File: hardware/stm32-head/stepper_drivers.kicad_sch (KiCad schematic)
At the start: 74 parts, among them J10 STEPPER4, J17 STEPPER6, J18 STEPPER5, J7 STEPPER1, J8 STEPPER2, J9 STEPPER3, U10 STSPIN220, U11 STSPIN220, U12 STSPIN220, U9 STSPIN220

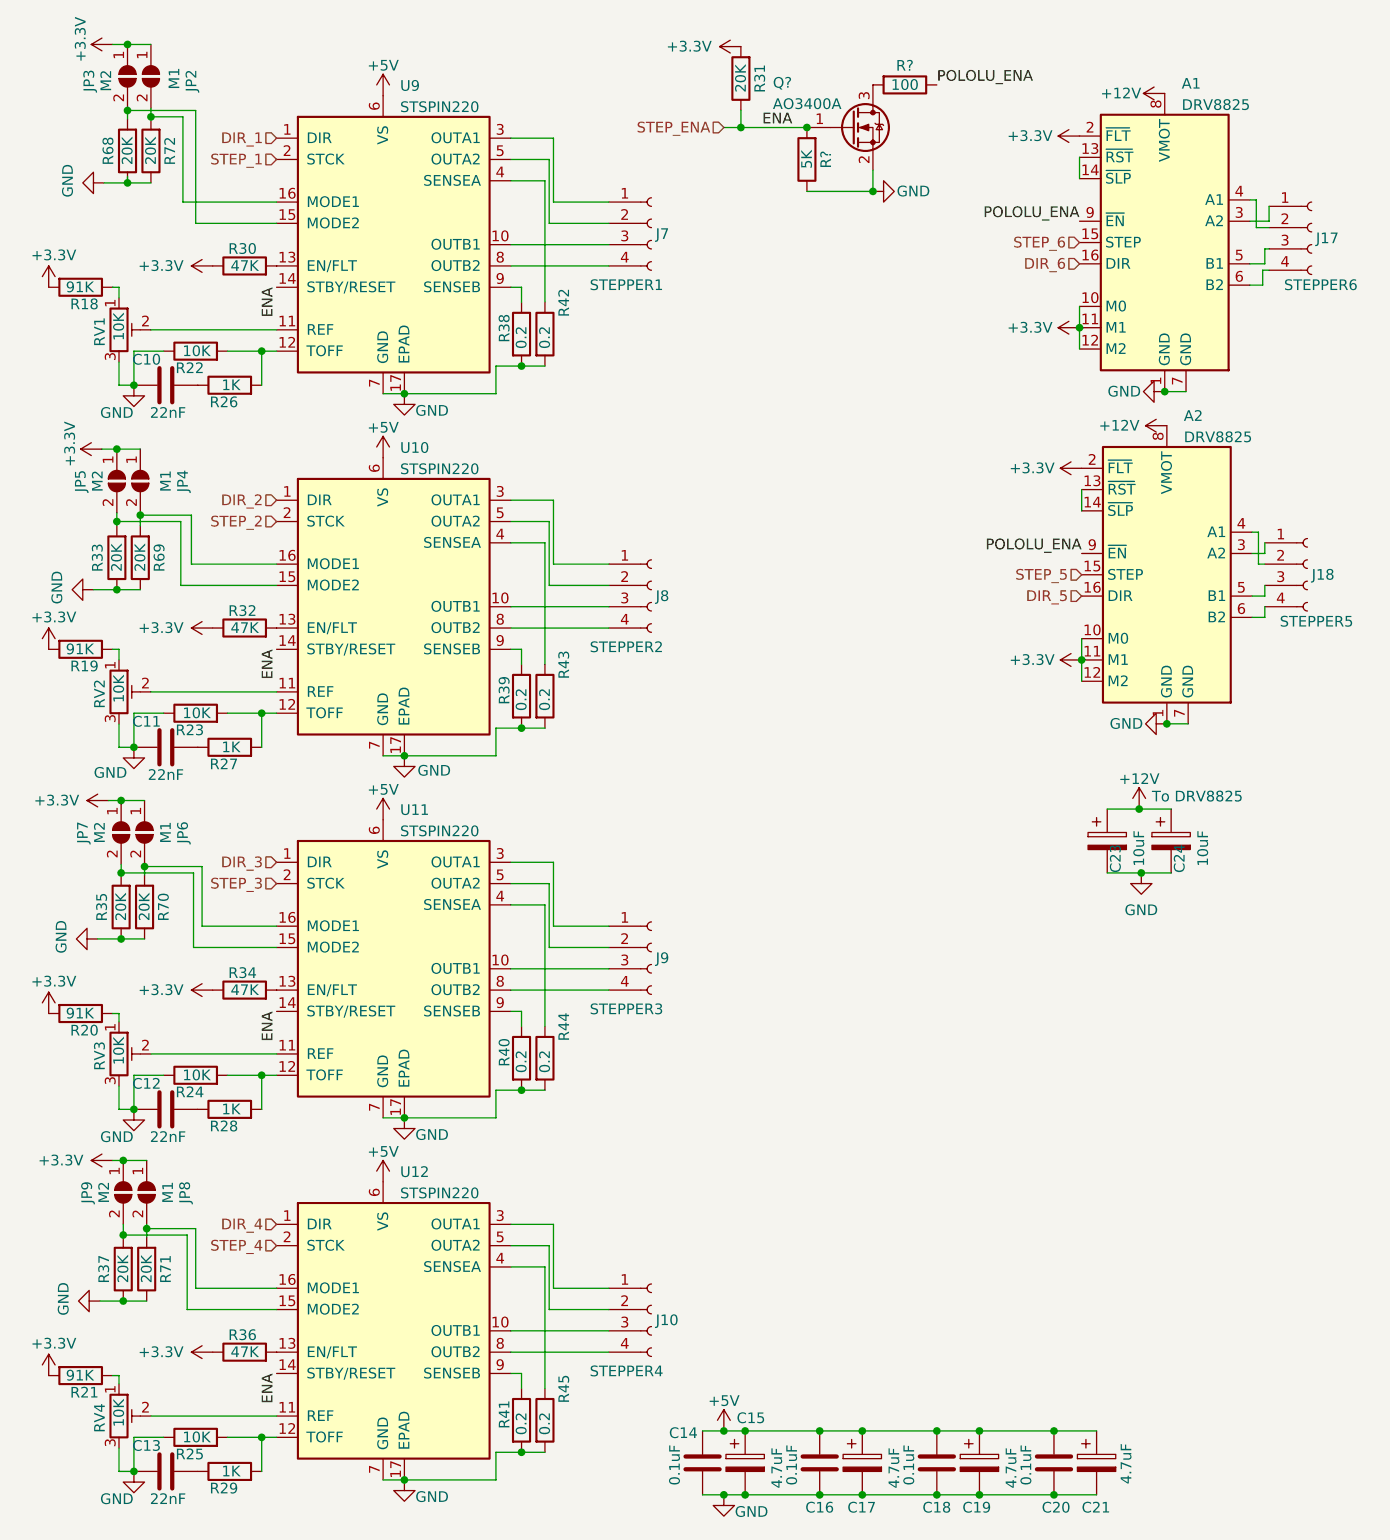
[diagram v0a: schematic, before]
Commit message: Some tweaks
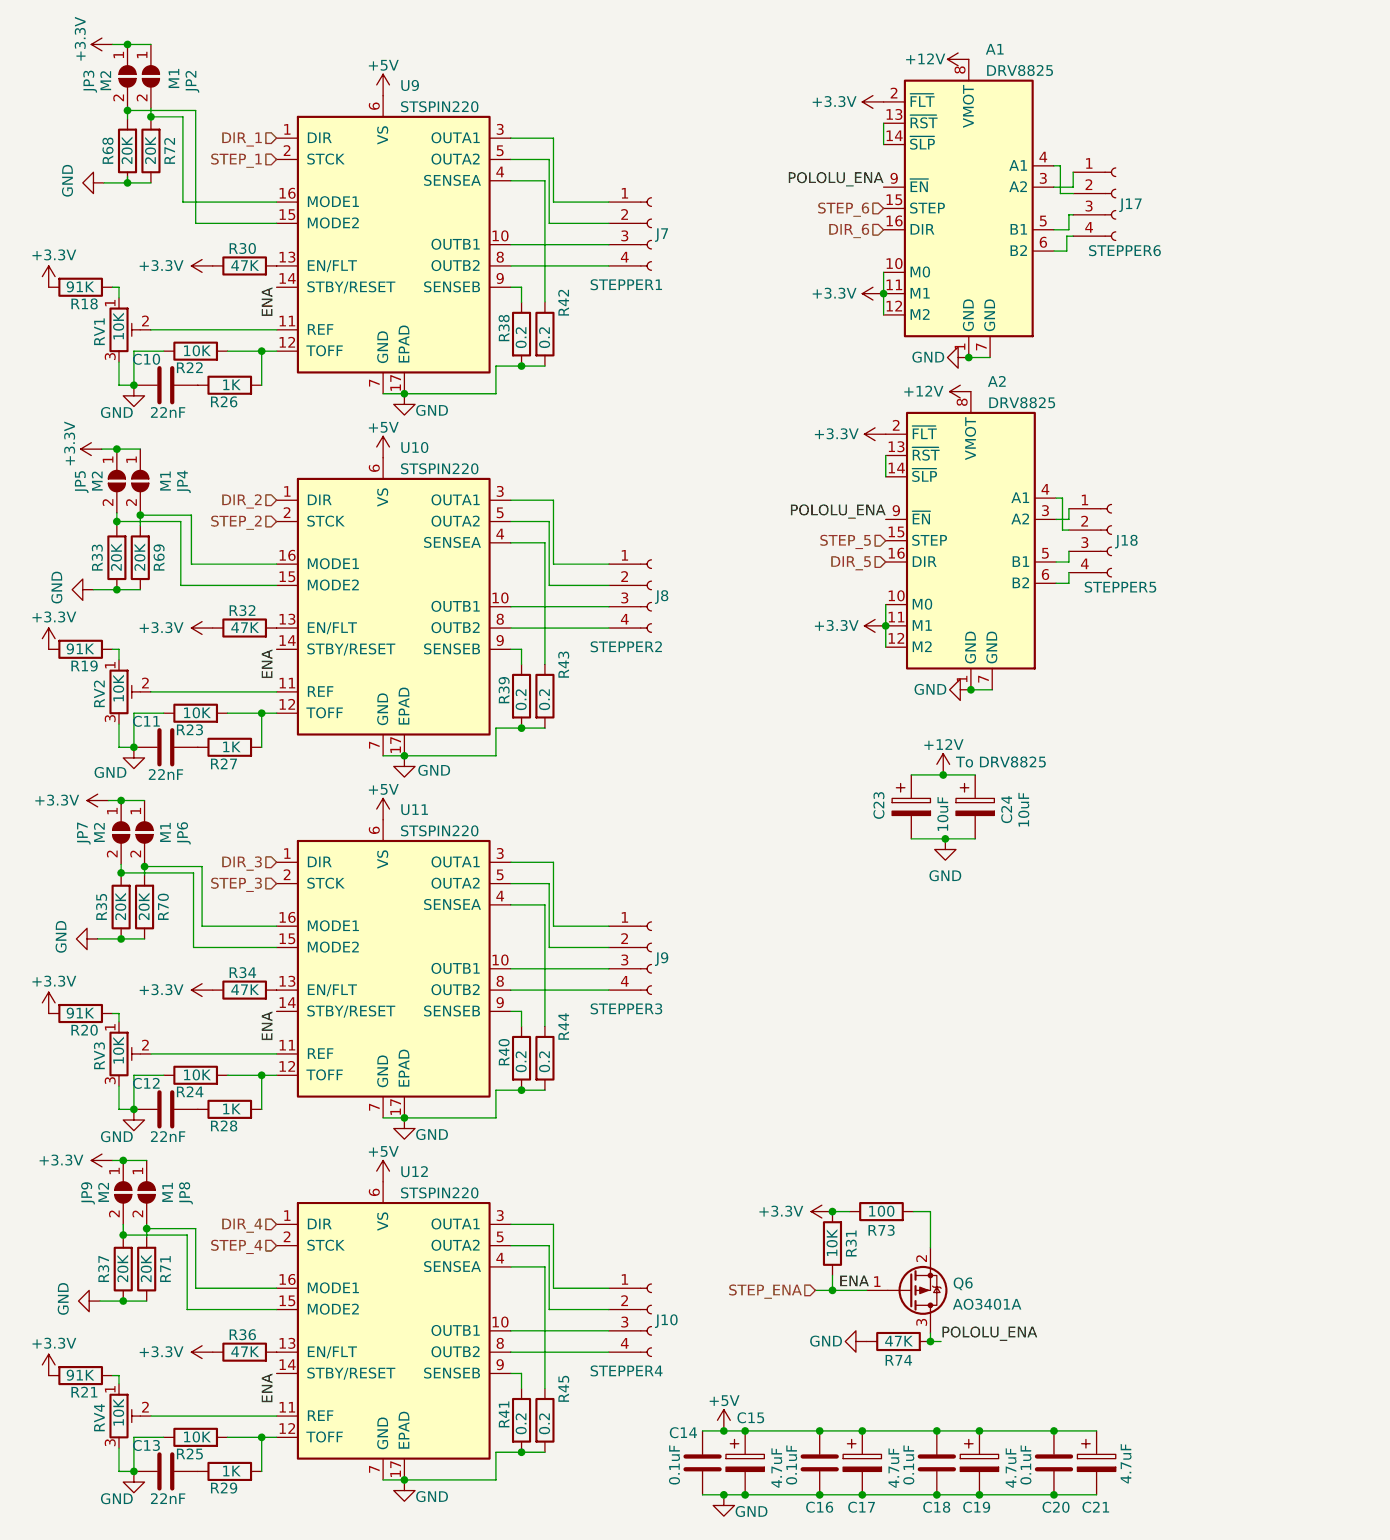
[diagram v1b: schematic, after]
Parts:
- removed Q?: AO3400A, Package_TO_SOT_SMD:SOT-23, symbol Transistor_FET:AO3400A
- removed R?: 5K, Resistor_SMD:R_0603_1608Metric, symbol Device:R
- added Q6: AO3401A, Package_TO_SOT_SMD:SOT-23, symbol Transistor_FET:AO3401A
- added R73: 100, Resistor_SMD:R_0603_1608Metric, symbol Device:R
- R31: value 20K -> 10K
- R74: renamed from R?; value 100 -> 47K
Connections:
- net +3.3V: now also R73.1
- net GND: now also R74.1
- net POLOLU_ENA: now also R74.2, Q6.3 (D); no longer R74.1
- net STEP_ENA: now also Q6.1 (G)
- new net: Q6.2 (S), R73.2
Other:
- moved on the sheet: A1, A2, C23, C24, J17, J18, R31, R74
